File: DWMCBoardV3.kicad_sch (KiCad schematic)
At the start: 7 parts, among them J1 Battery, J2 TPL5110, J3 MCU, Q1 S8050

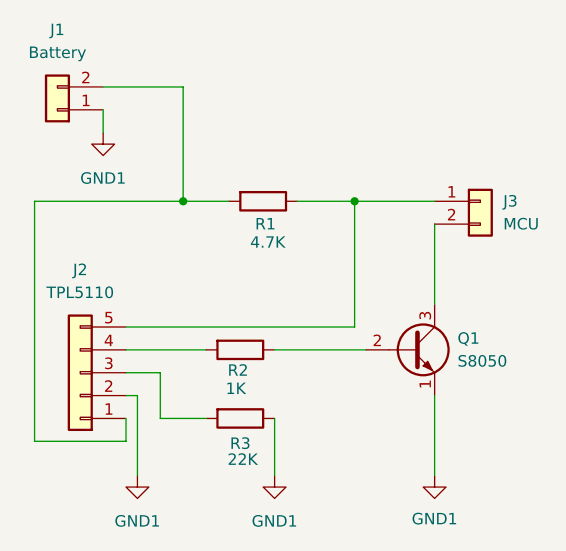
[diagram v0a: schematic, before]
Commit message: Add files via upload
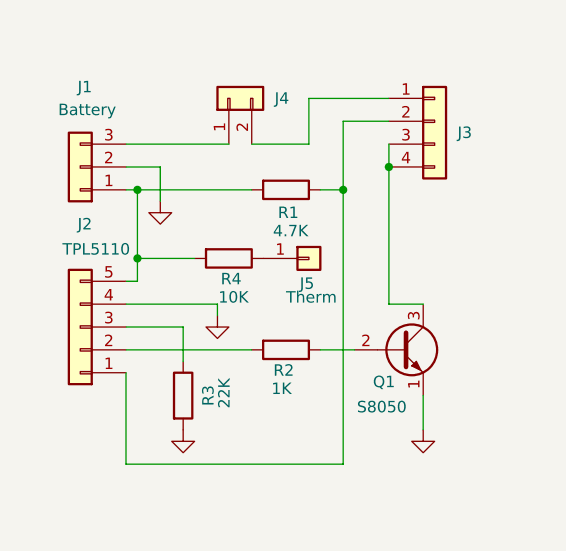
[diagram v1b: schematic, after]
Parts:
- removed J1: Battery, Connector_PinHeader_2.54mm:PinHeader_1x02_P2.54mm_Vertical, symbol Connector_Generic:Conn_01x02
- removed J3: MCU, Connector_PinHeader_2.54mm:PinHeader_1x02_P2.54mm_Vertical, symbol Connector_Generic:Conn_01x02
- added J1: Battery, Connector_PinHeader_2.54mm:PinHeader_1x03_P2.54mm_Vertical, symbol Connector_Generic:Conn_01x03
- added J3: Conn_01x04, Connector_PinHeader_2.54mm:PinHeader_1x04_P2.54mm_Vertical, symbol Connector_Generic:Conn_01x04
- added J4: Conn_01x02, Connector_PinHeader_2.54mm:PinHeader_1x02_P2.54mm_Vertical, symbol Connector_Generic:Conn_01x02
- added J5: Therm, Connector_PinHeader_2.54mm:PinHeader_1x01_P2.54mm_Vertical, symbol Connector_Generic:Conn_01x01
- added R4: 10K, Resistor_THT:R_Axial_DIN0207_L6.3mm_D2.5mm_P10.16mm_Horizontal, symbol Device:R
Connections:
- net at R2.2: now also J2.2 (Pin_2); no longer J2.4 (Pin_4)
- net at R1.1: now also J2.1 (Pin_1), J3.2 (Pin_2); no longer J2.5 (Pin_5)
- net at Q1.3 (C): now also J3.3 (Pin_3), J3.4 (Pin_4)
- net at R1.2: now also J2.5 (Pin_5), J1.1 (Pin_1), R4.2; no longer J2.1 (Pin_1)
- net at J2.3 (Pin_3): now also R3.1; no longer R3.2
- removed net GND1: J2.2 (Pin_2), Q1.1 (E), R3.1
- new net: J3.1 (Pin_1), J4.2 (Pin_2)
- new net: J1.3 (Pin_3), J4.1 (Pin_1)
- new net: J5.1 (Pin_1), R4.1
- new net GND: J1.2 (Pin_2), J2.4 (Pin_4), Q1.1 (E), R3.2
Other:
- moved on the sheet: J2, Q1, R1, R2, R3
